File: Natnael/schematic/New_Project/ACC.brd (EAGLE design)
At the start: 100 x 100 mm, 10 parts, among them J4 B2B-PH-K-S(LF)(SN)

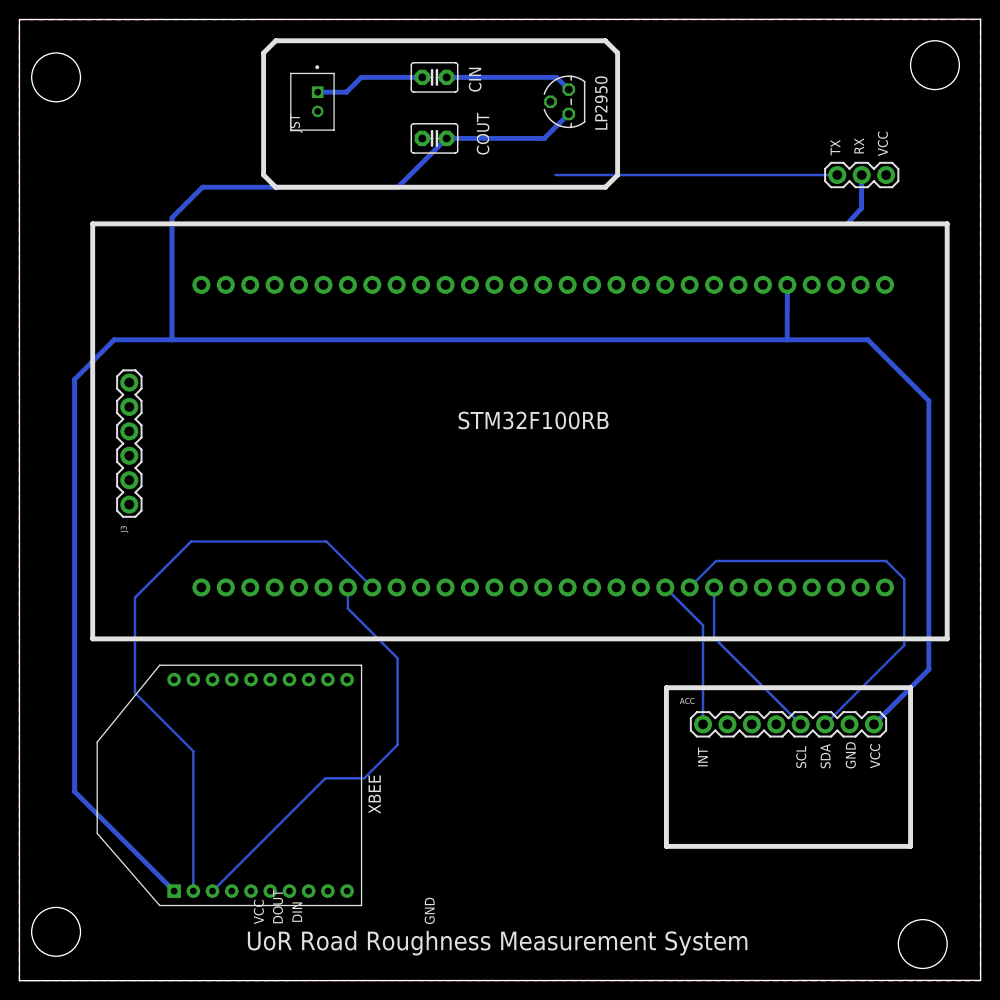
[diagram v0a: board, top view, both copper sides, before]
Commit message: updatae on pcb
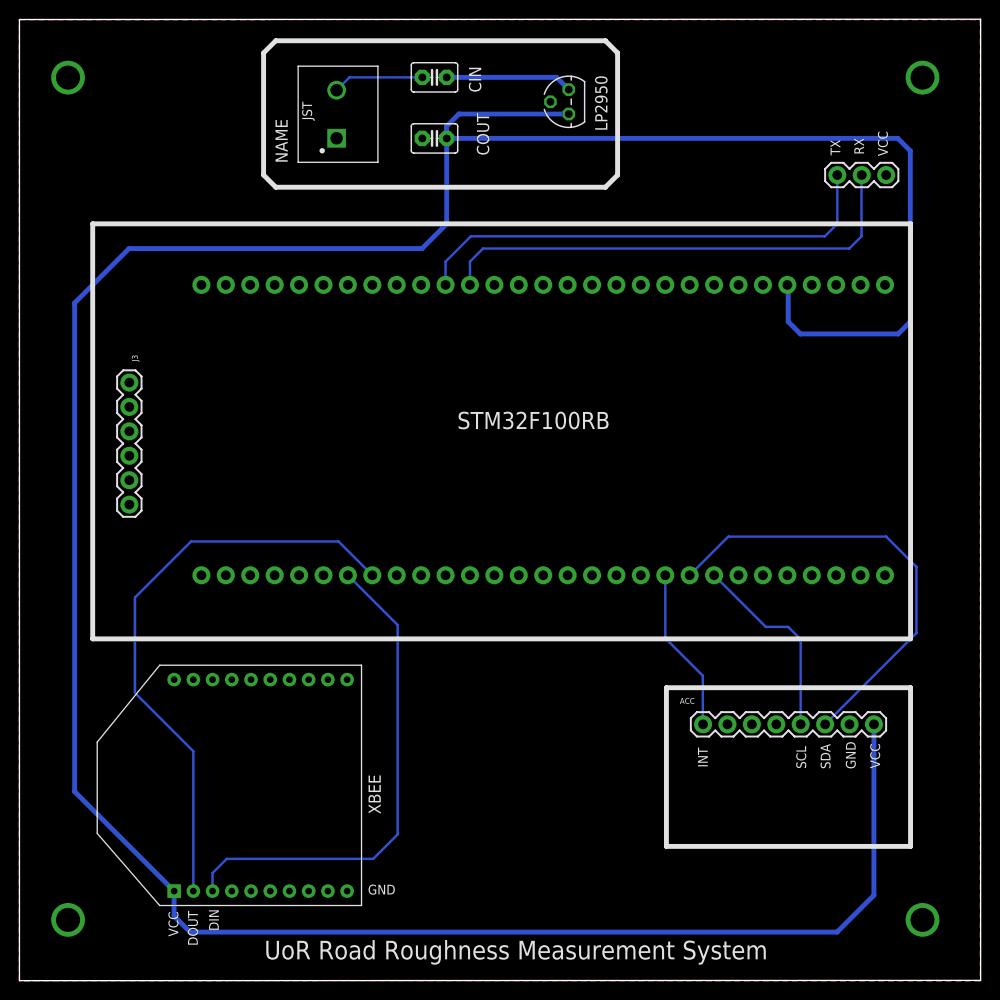
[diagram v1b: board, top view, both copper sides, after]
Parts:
- J4: value B2B-PH-K-S(LF)(SN) -> 1935161; device B2B-PH-K-S_LF__SN_:JST_B2B-PH-K-S(LF)(SN) -> 1935161:PHOENIX_1935161
- moved J3 12.7 mm to (11.5, 62.3), turned to 270 degrees
- moved J4 2.83 mm to (33.0, 90.2)
- moved J1 1.27 mm to (90.1, 42.2)
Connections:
- net GND: now also J4.1; no longer J4.2
- net N$1: now also J4.2; no longer J4.1
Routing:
- net 3V3: track 250.9 -> 310.6 mm
- net PA2: track 5.52 -> 50.6 mm
- net PA3: track 29.3 -> 49.9 mm
- net PA9: track 44.1 -> 51.9 mm
- net PB6: track 42.8 -> 46.9 mm
- net PB7: track 18.0 -> 20.6 mm
- net N$1: track 11.5 -> 9.47 mm
- net PB5: track 15.9 -> 17.1 mm
- net PA10: track 62.1 -> 61.6 mm
